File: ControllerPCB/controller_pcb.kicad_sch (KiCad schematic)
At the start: 2 parts, among them U1 Pico

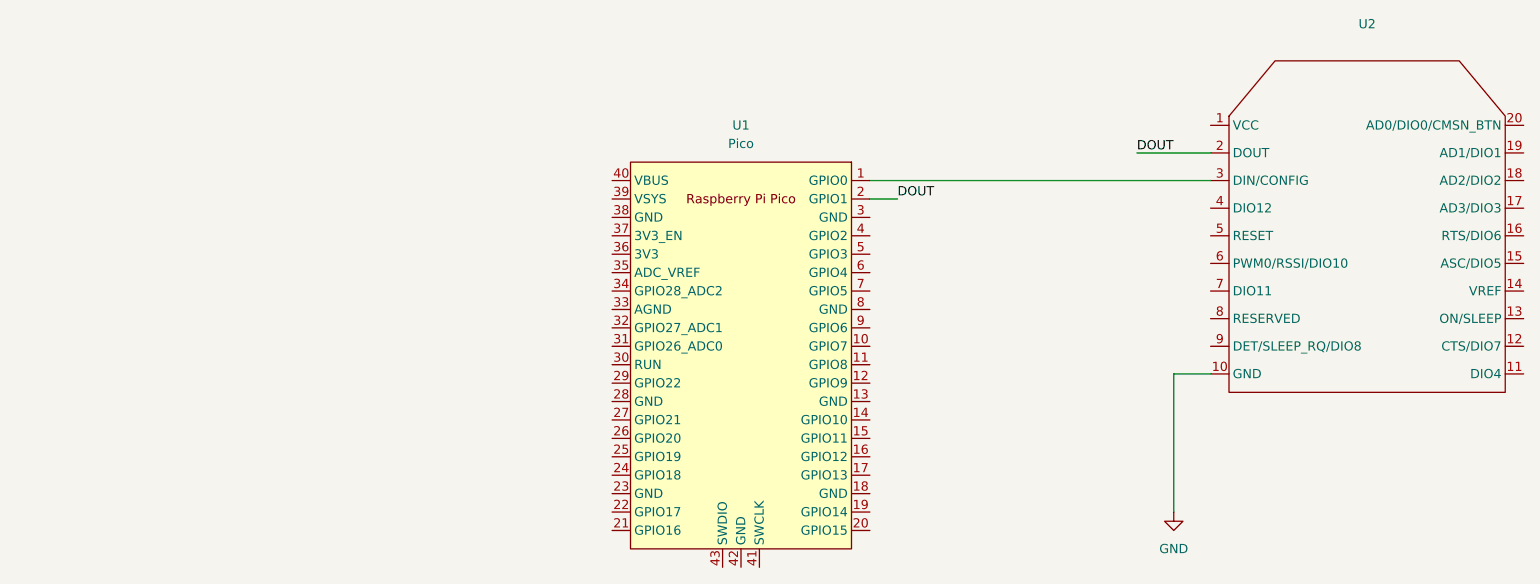
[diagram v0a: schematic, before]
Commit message: Add files via upload
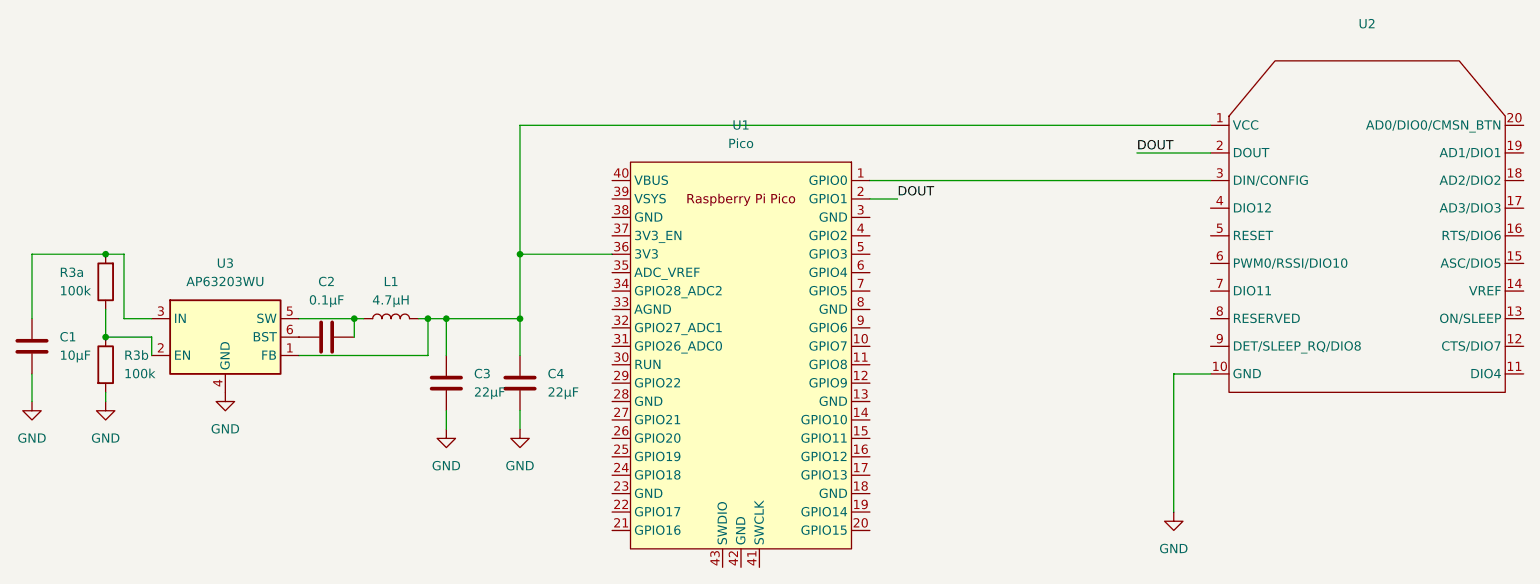
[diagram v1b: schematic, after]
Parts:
- added C1: 10µF, symbol Device:C
- added C2: 0.1µF, symbol Device:C
- added C3, C4: 22µF, symbol Device:C
- added L1: 4.7µH, symbol Device:L
- added R3a, R3b: 100k, symbol Device:R
- added U3: AP63203WU, Package_TO_SOT_SMD:TSOT-23-6, symbol Regulator_Switching:AP63203WU
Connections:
- net GND: now also C1.2, C3.2, C4.2, R3b.2, U3.4 (GND)
- net at U1.36 (3V3): now also U2.1 (VCC), C3.1, C4.1, L1.2, U3.1 (FB)
- new net: C2.2, L1.1, U3.5 (SW)
- new net: R3a.1, R3b.1, U3.2 (EN)
- new net: C1.1, R3a.2, U3.3 (IN)
- new net: C2.1, U3.6 (BST)
